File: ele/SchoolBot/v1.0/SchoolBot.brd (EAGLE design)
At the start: 95 x 60 mm, 58 parts, among them X1 M8, X2 M8, X4 POWER_IN

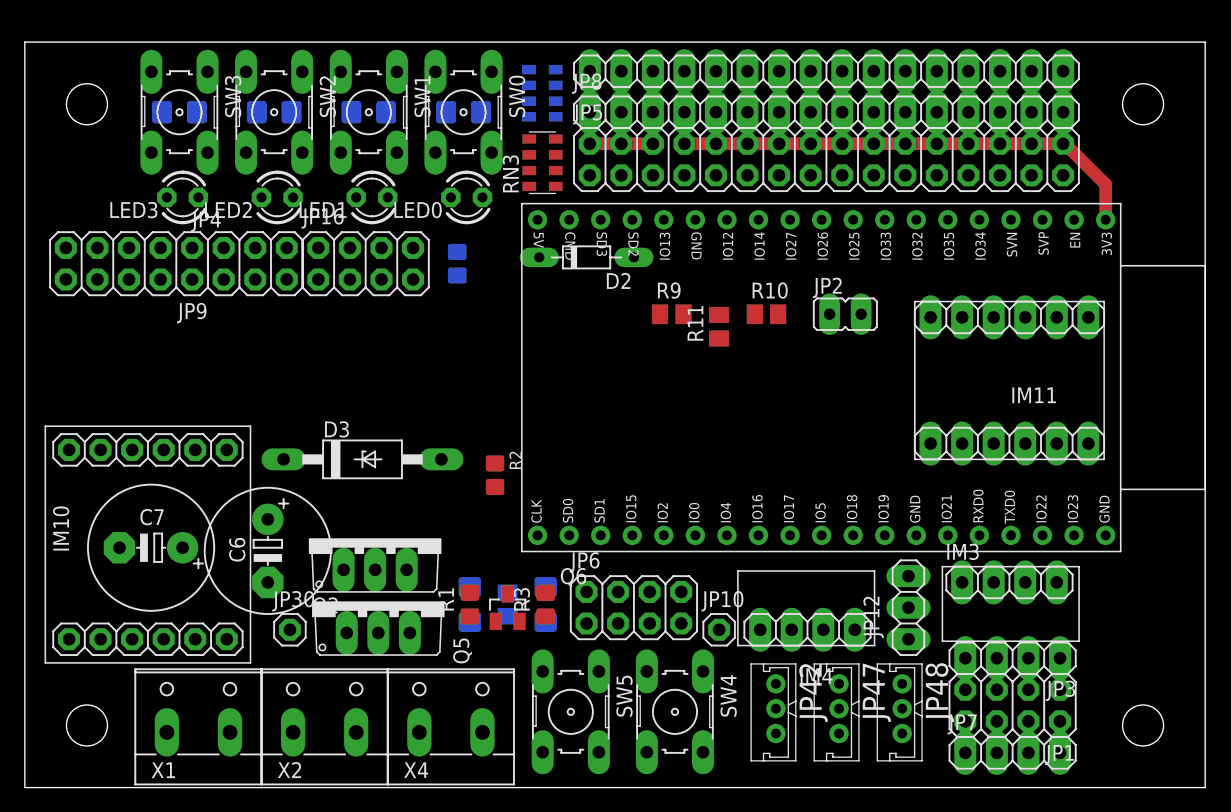
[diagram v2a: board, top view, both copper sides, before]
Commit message: new_board
nesting noveho rozlozeni
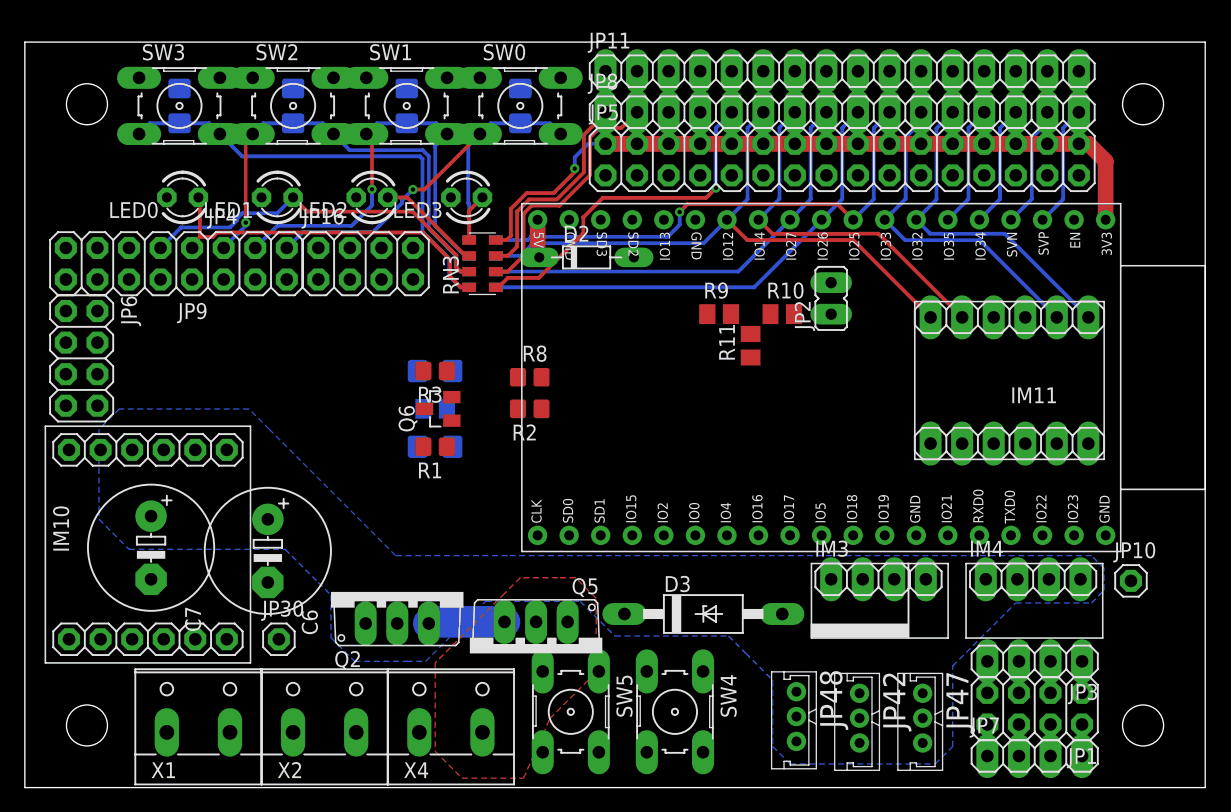
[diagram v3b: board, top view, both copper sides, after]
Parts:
- removed JP12: (no value), pinhead:1X03
- moved JP6 48.8 mm to (4.57, 34.5), turned to 270 degrees
- moved JP10 33.4 mm to (89.0, 16.6)
- moved D3 30.1 mm to (54.6, 14.0)
- moved LED0 22.9 mm to (12.7, 47.5)
- moved LED3 22.9 mm to (35.6, 47.5)
- moved C1 20.8 mm to (33.0, 33.5), turned to 180 degrees
- moved R3 20.8 mm to (33.0, 33.5), turned to 180 degrees
- moved Q6 16.9 mm to (33.3, 30.5), turned to 90 degrees
- moved R4 16.8 mm to (33.0, 30.5), turned to 180 degrees
- moved RN2 14.5 mm to (36.8, 42.2)
- moved Q5 13.4 mm to (41.1, 10.8), turned to 180 degrees
- moved C2 13.0 mm to (33.0, 27.4), turned to 0 degrees
- moved R1 13.0 mm to (33.0, 27.4), turned to 180 degrees
- moved R8 10.9 mm to (40.6, 33.0), flipped to the top, turned to 0 degrees
- moved IM3 10.5 mm to (63.6, 18.0)
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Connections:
- net N$7 renamed ON
- removed net N$5: JP9.10, JP9.2, JP9.4, JP9.6, JP9.8
- removed net N$6: IM6.2
- net +5V: no longer JP1.2, JP1.4, JP1.6, JP1.8
- net EN: now also IM6.2
- net ENC_B1: now also IM6.31; no longer IM6.23
- net ENC_B2: now also IM6.23; no longer IM6.31
- net GND: now also JP9.10, JP9.2, JP9.4, JP9.6, JP9.8; no longer JP12.1
- net GPIO12: now also IM11.6, JP11.6, JP8.6; no longer IM11.2, JP11.1, JP8.1
- net GPIO14: now also IM11.5, JP11.7, JP8.7; no longer IM11.1, JP11.2, JP8.2
- net GPIO14-5V: no longer JP12.3
- net GPIO22: now also JP11.2, JP8.2; no longer JP11.6, JP8.6
- net GPIO23: now also JP11.1, JP8.1; no longer JP11.7, JP8.7
- net GPIO25: now also JP11.10, JP8.10; no longer JP11.8, JP8.8
- net GPIO27: now also JP11.8, JP8.8; no longer JP11.10, JP8.10
- net GPIO32: now also IM11.1, JP11.12, JP8.12; no longer IM11.6, JP11.11, JP8.11
- net GPIO33: now also IM11.2, JP11.11, JP8.11; no longer IM11.5, JP11.12, JP8.12
- net GPIO34: now also JP11.14, JP8.14; no longer JP11.13, JP8.13
- net GPIO35: now also JP11.13, JP8.13; no longer JP11.14, JP8.14
- net GPIO36: now also JP11.16, JP8.16; no longer JP11.15, JP8.15
- net GPIO39: now also JP11.15, JP8.15; no longer JP11.16, JP8.16
- net SERVO_STEPDOWN_5V: now also JP1.2, JP1.4, JP1.6, JP1.8; no longer JP12.2
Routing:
- net GPIO12: track 0.00 -> 52.6 mm
- net GPIO25: track 0.00 -> 44.3 mm, vias 0 -> 1
- net GPIO26: track 0.00 -> 41.7 mm
- net GPIO27: track 0.00 -> 38.6 mm
- net SW2: track 0.00 -> 36.8 mm, vias 0 -> 1
- net SW3: track 0.00 -> 36.7 mm
- net SW0: track 0.00 -> 35.6 mm, vias 0 -> 1
- net SW1: track 0.00 -> 35.5 mm, vias 0 -> 1
- net GPIO14: track 0.00 -> 32.8 mm
- net GPIO21: track 0.00 -> 31.7 mm, vias 0 -> 1
- net GPIO32: track 0.00 -> 30.3 mm
- net GPIO33: track 0.00 -> 30.3 mm
- net LED1: track 0.00 -> 29.6 mm
- net LED0: track 0.00 -> 28.8 mm
- net GPIO22: track 0.00 -> 23.7 mm
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- added copper zone on layer 1, net BAT1
- added copper zone on layer 16, net VCC
